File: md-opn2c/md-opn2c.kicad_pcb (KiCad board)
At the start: 2 copper layers, 53.1 x 29.4 mm, 41 parts, among them U1 TL072, U2 74HCT08, U3 YM3438

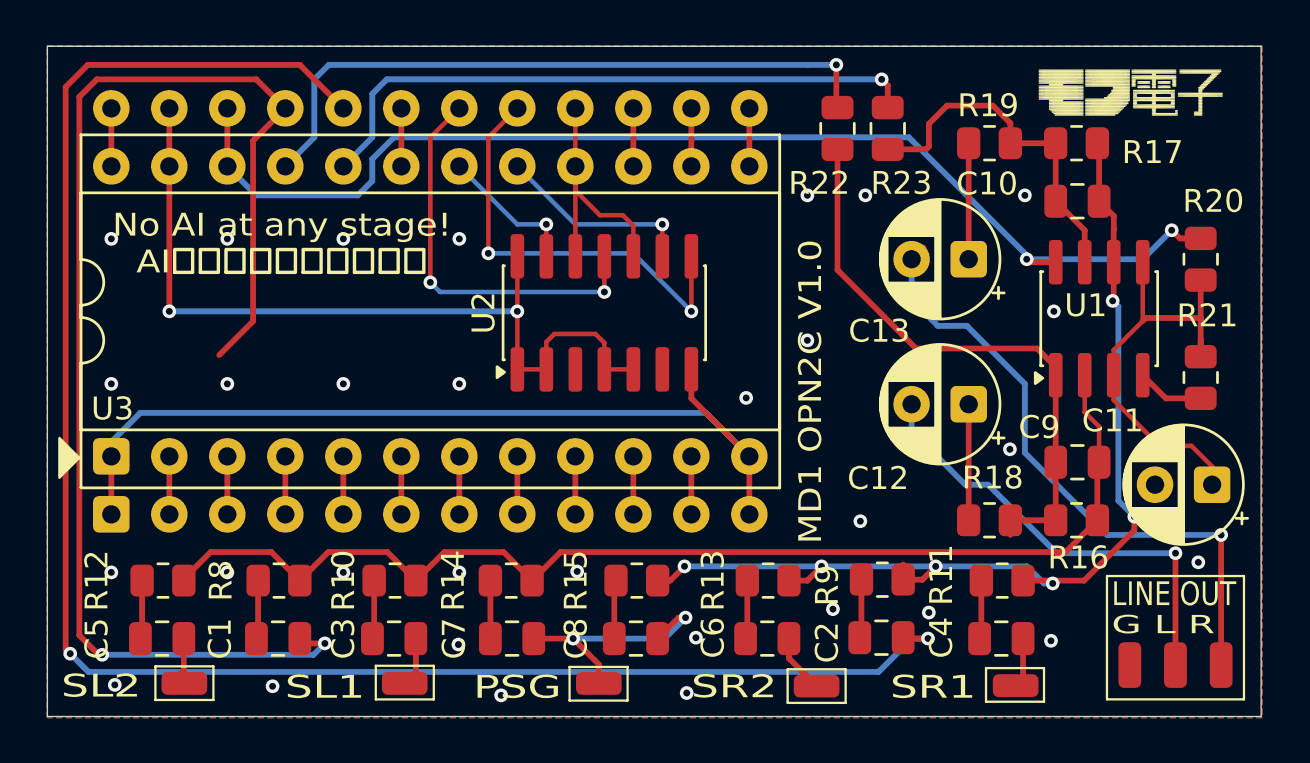
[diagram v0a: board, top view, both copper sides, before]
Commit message: Updated readme for upcoming V1.0.1 revision
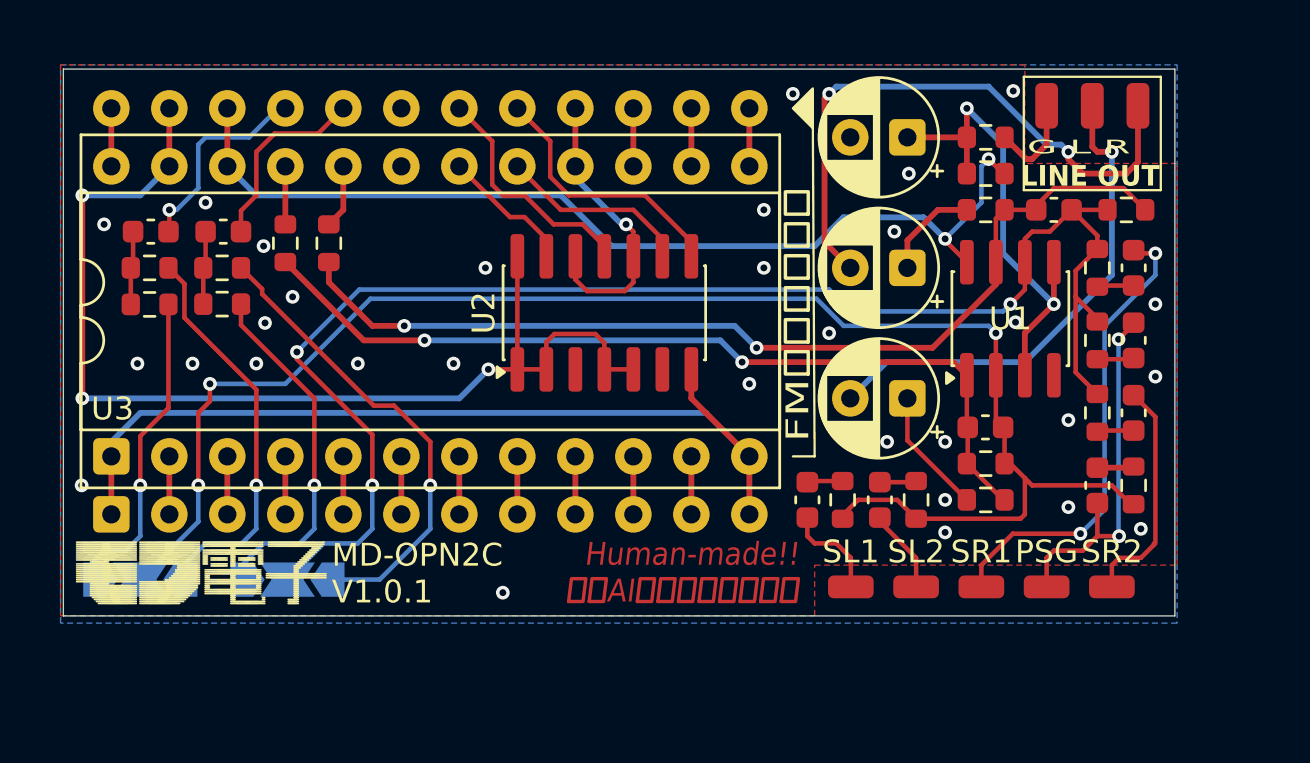
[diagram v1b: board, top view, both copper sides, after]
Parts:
- added JP1: SolderJumper_3_Open, Jumper:SolderJumper-3_P2.0mm_Open_TrianglePad1.0x1.5mm, B.Cu at (26.7, 41.0)
- added JP2: SolderJumper_3_Open, Jumper:SolderJumper-3_P2.0mm_Open_TrianglePad1.0x1.5mm, B.Cu at (33.1, 41.0)
- added R24: 10k, Resistor_SMD:R_0603_1608Metric, F.Cu at (27.1, 28.9)
- added R25: 10k, Resistor_SMD:R_0603_1608Metric, F.Cu at (30.3, 28.9)
- C1, C10, C2, C3, C4, C5, C6, C7, C8, C9: footprint Capacitor_SMD:C_0805_2012Metric -> Capacitor_SMD:C_0603_1608Metric
- JOPN1: value YM2612 Socket -> DIP24 Header
- R10, R11, R12, R13, R14, R15, R16, R17, R18, R19, R20, R21, R22, R23, R8, R9: footprint Resistor_SMD:R_0805_2012Metric -> Resistor_SMD:R_0603_1608Metric
- U1: value TL072 -> TL972
- moved C2 33.9 mm to (30.3, 25.7)
- moved R12 33.2 mm to (60.6, 37.5), turned to -90 degrees
- moved IN_SL2 32.3 mm to (60.6, 41.3)
- moved C5 32.0 mm to (59.1, 37.5), turned to 90 degrees
- moved R9 32.0 mm to (30.3, 27.3)
- moved R14 27.6 mm to (70.2, 36.8), turned to -90 degrees
- moved C7 26.5 mm to (68.6, 36.8), turned to 90 degrees
- moved C8 25.4 mm to (70.2, 30.5), turned to -90 degrees
- moved R23 25.0 mm to (34.9, 26.2)
- moved OUT_GND1 24.8 mm to (66.4, 20.2), turned to 180 degrees
- moved OUT_L1 24.8 mm to (68.4, 20.2), turned to 180 degrees
- moved OUT_R1 24.8 mm to (70.4, 20.2), turned to 180 degrees
- moved R22 24.7 mm to (33.0, 26.2)
- moved R15 22.7 mm to (68.6, 30.5), turned to 90 degrees
- moved C11 20.2 mm to (60.3, 21.6)
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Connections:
- R8 pad 2: /MIX_L -> Net-(JP1-B)
- R9 pad 2: /MIX_R -> Net-(JP2-B)
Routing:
- net /OPN2C_MOR: track 77.9 -> 8.37 mm, vias 2 -> 0
- net /OPN2C_MOL: track 58.0 -> 9.01 mm, vias 2 -> 1
- net /BUF_R: track 15.7 -> 42.9 mm, vias 0 -> 2
- net /ORIG_OUT_L: track 29.4 -> 2.54 mm, vias 1 -> 0
- net /ORIG_OUT_R: track 27.6 -> 2.80 mm, vias 1 -> 0
- net Net-(JP2-B): track 0.00 -> 20.6 mm, vias 0 -> 1
- net /MIX_R: track 45.5 -> 64.7 mm, vias 6 -> 3
- net /SR1: track 2.19 -> 20.5 mm, vias 0 -> 2
- net /MIX_L: track 50.9 -> 69.1 mm, vias 0 -> 3
- net Net-(JP1-B): track 0.00 -> 17.5 mm, vias 0 -> 1
- net Net-(JP2-A): track 0.00 -> 16.1 mm, vias 0 -> 1
- net Net-(JP1-A): track 0.00 -> 13.9 mm, vias 0 -> 1
- net /BUF_L: track 26.0 -> 38.1 mm, vias 0 -> 2
- net VCC: track 36.8 -> 48.0 mm, vias 2 -> 3
- net VCCA: track 51.6 -> 43.0 mm
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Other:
- board size 53.1 x 29.4 mm -> 48.7 x 23.9 mm
- board text added: "FM音源をここに"
- board text added: "Human-made!! 全くAI利用していません"
- board text added: "Jumpers: YM2612 YM3438"
- board text added: "MD-OPN2C V1.0.1"
- board text removed: "MD1 OPN2C V1.0"
- board text removed: "No AI at any stage! AI全く利用していないよ"
